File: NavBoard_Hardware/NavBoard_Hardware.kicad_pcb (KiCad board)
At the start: 2 copper layers, 61 x 100 mm, 61 parts, among them J1 Conn_Coaxial, Q1 BSS138, Q2 BSS138, U2 ATMEGA328P-Project_Library, U3 OKI, U4 OKI, U5 FGPMMOPA6H, Y1 Crystal

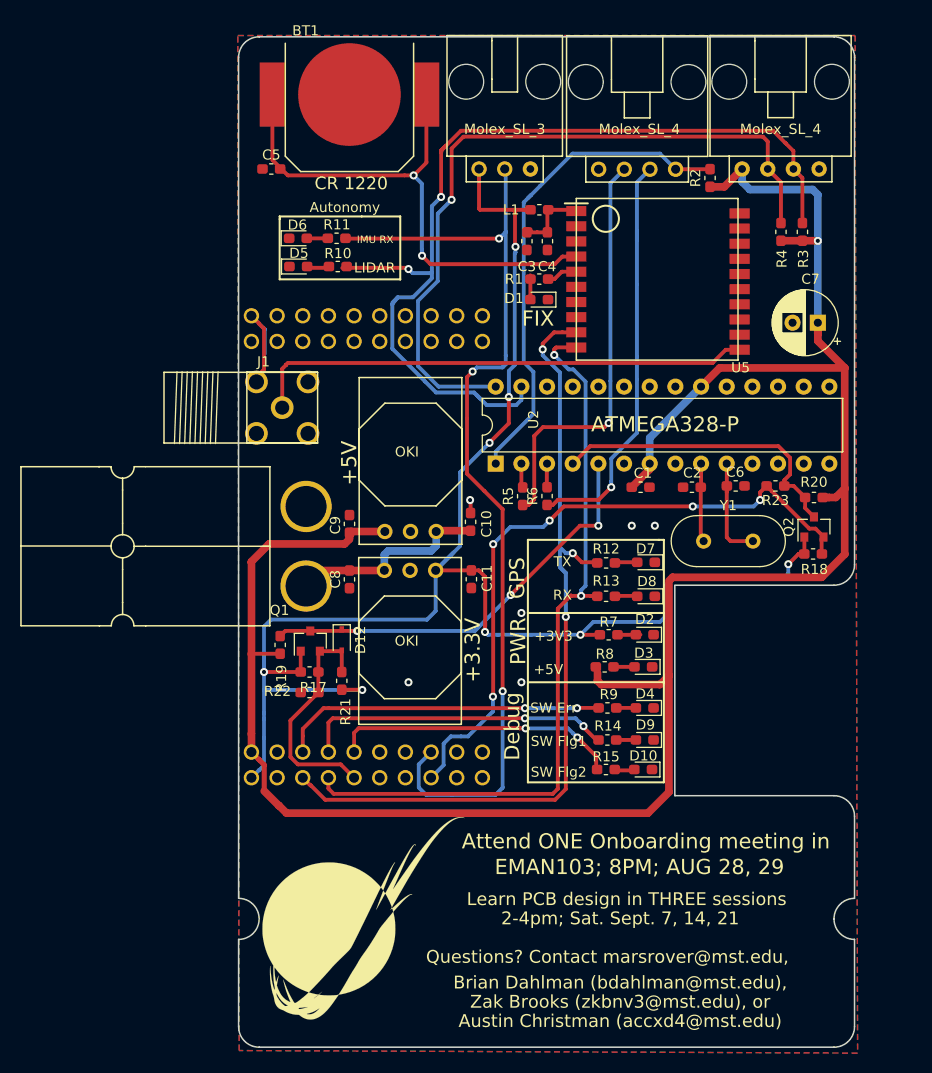
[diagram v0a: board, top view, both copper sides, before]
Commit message: revision 1
made some text changes
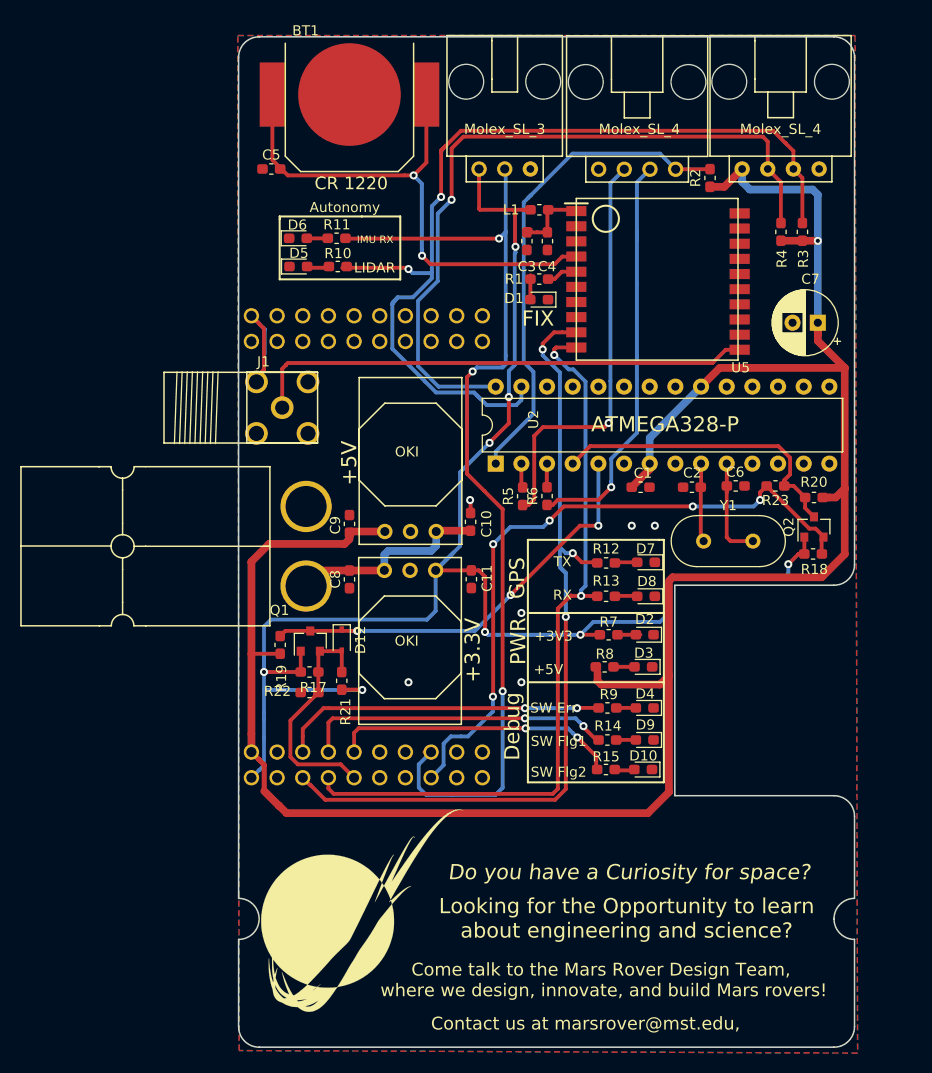
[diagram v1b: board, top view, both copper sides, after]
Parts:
- moved G*** 0.77 mm to (127.5, 138.9)
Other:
- board text added: "Come talk to the Mars Rover Design Team, where we design, innovate, and build Mars rovers!"
- board text added: "Contact us at marsrover@mst.edu,"
- board text added: "Do you have a Curiosity for space?"
- board text added: "Looking for the Opportunity to learn about engineering and science?"
- board text removed: "2-4pm; Sat. Sept. 7, 14, 21"
- board text removed: "Attend ONE Onboarding meeting in"
- board text removed: "Austin Christman (accxd4@mst.edu)"
- board text removed: "Brian Dahlman (bdahlman@mst.edu),"
- board text removed: "EMAN103; 8PM; AUG 28, 29"
- board text removed: "Learn PCB design in THREE sessions"
- board text removed: "Questions? Contact marsrover@mst.edu,"
- board text removed: "Zak Brooks (zkbnv3@mst.edu), or"
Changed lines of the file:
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@@
-(kicad_pcb (version 20171130) (host pcbnew "(5.0.0)")
+(kicad_pcb (version 20171130) (host pcbnew "(5.1.2)-1")
   (general
     (thickness 1.6)
-    (drawings 70)
+    (drawings 66)
     (tracks 508)
     (zones 0)
@@
     (zone_45_only no)
     (trace_min 0.2)
-    (segment_width 0.2)
-    (edge_width 0.15)
     (via_size 0.8)
     (via_drill 0.4)
@@
     (uvia_min_size 0.2)
     (uvia_min_drill 0.1)
+    (edge_width 0.15)
+    (segment_width 0.2)
     (pcb_text_width 0.3)
     (pcb_text_size 1.5 1.5)
@@
   )
   (module MRDT_Silkscreens:MRDT_Logo_20mm (layer F.Cu)
-    (at 127.635 139.7)
+    (at 127.508 138.938)
     (tags "Logo, MRDT")
     (fp_text reference G*** (at -3.6068 11.8364) (layer Dwgs.User) hide
@@
       (xy 12.275375 35.246544) (xy 12.443517 35.256332) (xy 12.564924 35.258447) (xy 12.646643 35.249446)) (layer B.SilkS) (width 0.01))
   )
+  (gr_line (start 176.2252 104.6988) (end 176.2252 54.483) (layer Edge.Cuts) (width 0.15))
   (gr_text Molex_SL_4 (at 168.91 61.595) (layer F.SilkS)
     (effects (font (size 1.016 1.016) (thickness 0.127)))
@@
     (effects (font (size 2.54 2.921) (thickness 0.508)) (justify mirror))
   )
-  (gr_text "Zak Brooks (zkbnv3@mst.edu), or" (at 153.035 147.955) (layer F.SilkS)
+  (gr_text "Contact us at marsrover@mst.edu,\n" (at 149.606 150.114) (layer F.SilkS)
     (effects (font (size 1.27 1.27) (thickness 0.3)))
   )
-  (gr_text "Austin Christman (accxd4@mst.edu)" (at 153.035 149.86) (layer F.SilkS)
-    (effects (font (size 1.27 1.27) (thickness 0.3)))
-  )
-  (gr_text "Brian Dahlman (bdahlman@mst.edu), \n" (at 153.035 146.05) (layer F.SilkS)
-    (effects (font (size 1.27 1.27) (thickness 0.3)))
-  )
-  (gr_text "Questions? Contact marsrover@mst.edu,\n" (at 151.765 143.51) (layer F.SilkS)
-    (effects (font (size 1.27 1.27) (thickness 0.3)))
-  )
-  (gr_text "2-4pm; Sat. Sept. 7, 14, 21\n" (at 153.035 139.7) (layer F.SilkS)
-    (effects (font (size 1.27 1.27) (thickness 0.3)))
-  )
-  (gr_text "EMAN103; 8PM; AUG 28, 29 " (at 154.94 134.62) (layer F.SilkS)
+  (gr_text "Looking for the Opportunity to learn \nabout engineering and science?" (at 153.67 139.7) (layer F.SilkS)
     (effects (font (size 1.5 1.5) (thickness 0.3)))
   )
-  (gr_text "Attend ONE Onboarding meeting in " (at 155.575 132.08) (layer F.SilkS)
-    (effects (font (size 1.5 1.5) (thickness 0.3)))
+  (gr_text "Do you have a Curiosity for space?" (at 153.924 135.128) (layer F.SilkS)
+    (effects (font (size 1.5 1.5) (thickness 0.3) italic))
   )
-  (gr_text "Learn PCB design in THREE sessions " (at 153.67 137.795) (layer F.SilkS)
+  (gr_text "Come talk to the Mars Rover Design Team,\n where we design, innovate, and build Mars rovers!" (at 151.13 145.796) (layer F.SilkS)
     (effects (font (size 1.27 1.27) (thickness 0.3)))
   )
@@
     (effects (font (size 1.5 1.5) (thickness 0.3)))
   )
-  (gr_line (start 158.468 106.7308) (end 174.1906 106.7308) (layer Edge.Cuts) (width 0.15))
+  (gr_line (start 158.4452 106.7308) (end 174.1932 106.7308) (layer Edge.Cuts) (width 0.15))
   (gr_line (start 143.8965 109.474) (end 143.8965 102.235) (layer F.SilkS) (width 0.2))
   (gr_line (start 143.8965 126.238) (end 143.8965 109.474) (layer F.SilkS) (width 0.2))
@@
   (gr_line (start 158.4452 127.5588) (end 174.1932 127.5588) (layer Edge.Cuts) (width 0.15))
   (gr_line (start 158.4452 106.7308) (end 158.4452 127.5588) (layer Edge.Cuts) (width 0.15))
-  (gr_line (start 176.2252 54.483) (end 176.2252 104.6988) (layer Edge.Cuts) (width 0.15))
   (gr_line (start 117.2972 52.451) (end 174.1932 52.451) (layer Edge.Cuts) (width 0.15))
   (gr_arc (start 117.2972 54.483) (end 117.2972 52.451) (angle -90) (layer Edge.Cuts) (width 0.15))

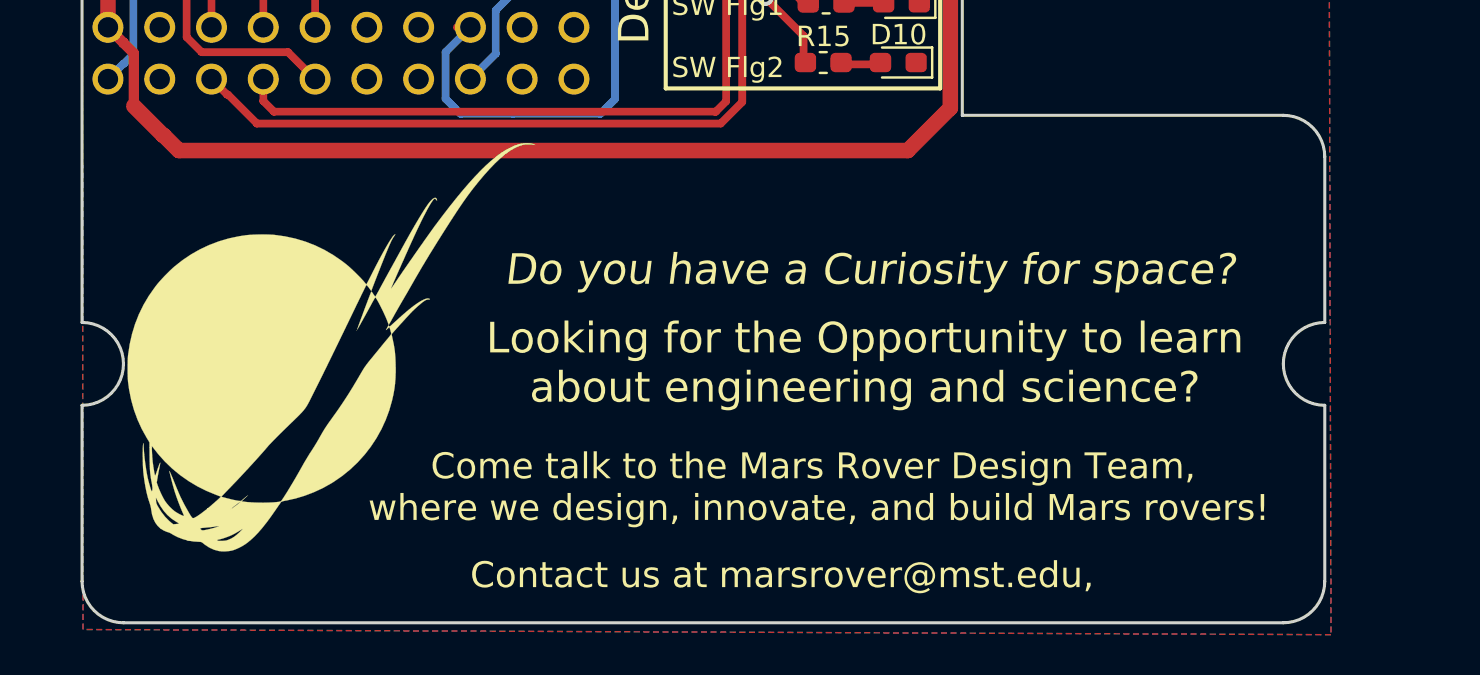
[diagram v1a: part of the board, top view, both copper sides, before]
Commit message: rev2
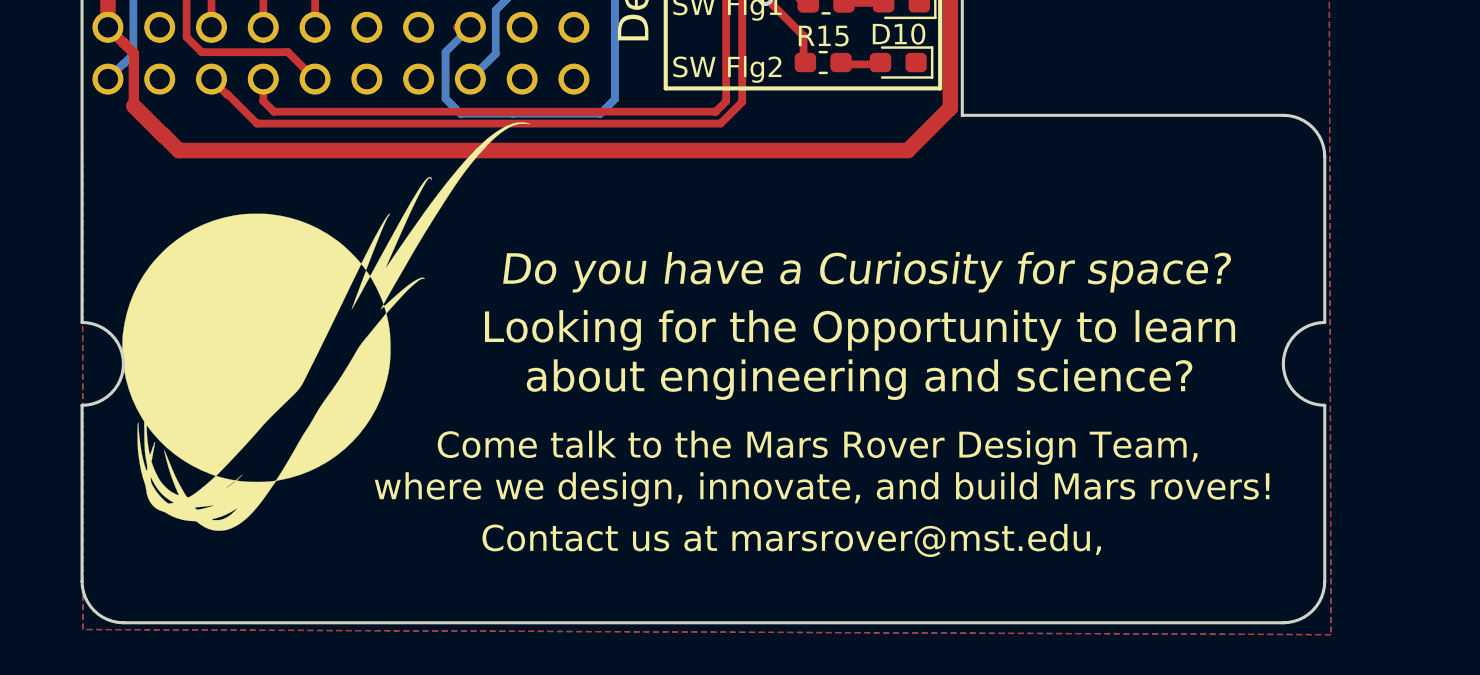
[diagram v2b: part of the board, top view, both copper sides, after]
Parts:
- moved G*** 1.05 mm to (127.3, 137.9)
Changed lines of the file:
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@@
   )
   (module MRDT_Silkscreens:MRDT_Logo_20mm (layer F.Cu)
-    (at 127.508 138.938)
+    (at 127.254 137.922)
     (tags "Logo, MRDT")
     (fp_text reference G*** (at -3.6068 11.8364) (layer Dwgs.User) hide
@@
     (effects (font (size 2.54 2.921) (thickness 0.508)) (justify mirror))
   )
-  (gr_text "Contact us at marsrover@mst.edu,\n" (at 149.606 150.114) (layer F.SilkS)
+  (gr_text "Contact us at marsrover@mst.edu,\n" (at 150.114 148.336) (layer F.SilkS)
     (effects (font (size 1.27 1.27) (thickness 0.3)))
   )
-  (gr_text "Looking for the Opportunity to learn \nabout engineering and science?" (at 153.67 139.7) (layer F.SilkS)
+  (gr_text "Looking for the Opportunity to learn \nabout engineering and science?" (at 153.416 139.192) (layer F.SilkS)
     (effects (font (size 1.5 1.5) (thickness 0.3)))
   )
-  (gr_text "Do you have a Curiosity for space?" (at 153.924 135.128) (layer F.SilkS)
+  (gr_text "Do you have a Curiosity for space?" (at 153.67 135.128) (layer F.SilkS)
     (effects (font (size 1.5 1.5) (thickness 0.3) italic))
   )
-  (gr_text "Come talk to the Mars Rover Design Team,\n where we design, innovate, and build Mars rovers!" (at 151.13 145.796) (layer F.SilkS)
+  (gr_text "Come talk to the Mars Rover Design Team,\n where we design, innovate, and build Mars rovers!" (at 151.384 144.78) (layer F.SilkS)
     (effects (font (size 1.27 1.27) (thickness 0.3)))
   )
